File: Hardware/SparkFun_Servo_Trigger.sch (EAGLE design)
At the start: 30 parts, among them U1 ATTINY84, Y1 16MHZ

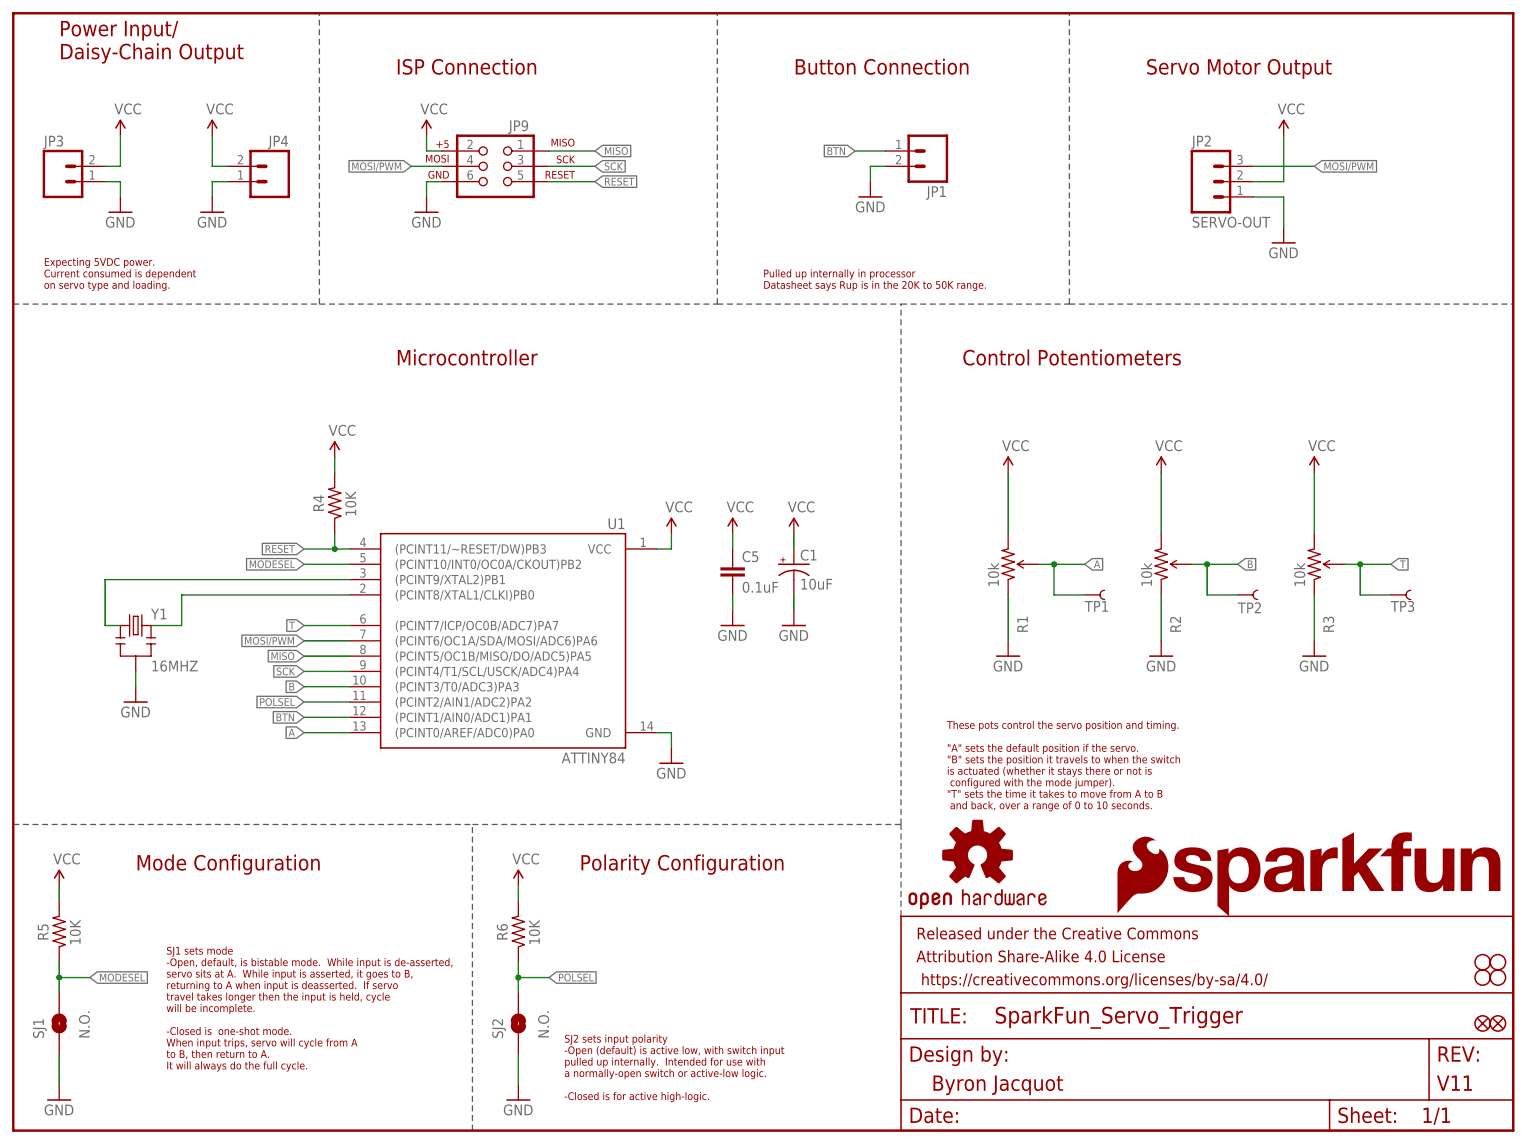
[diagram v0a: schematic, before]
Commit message: Updates from checklist.
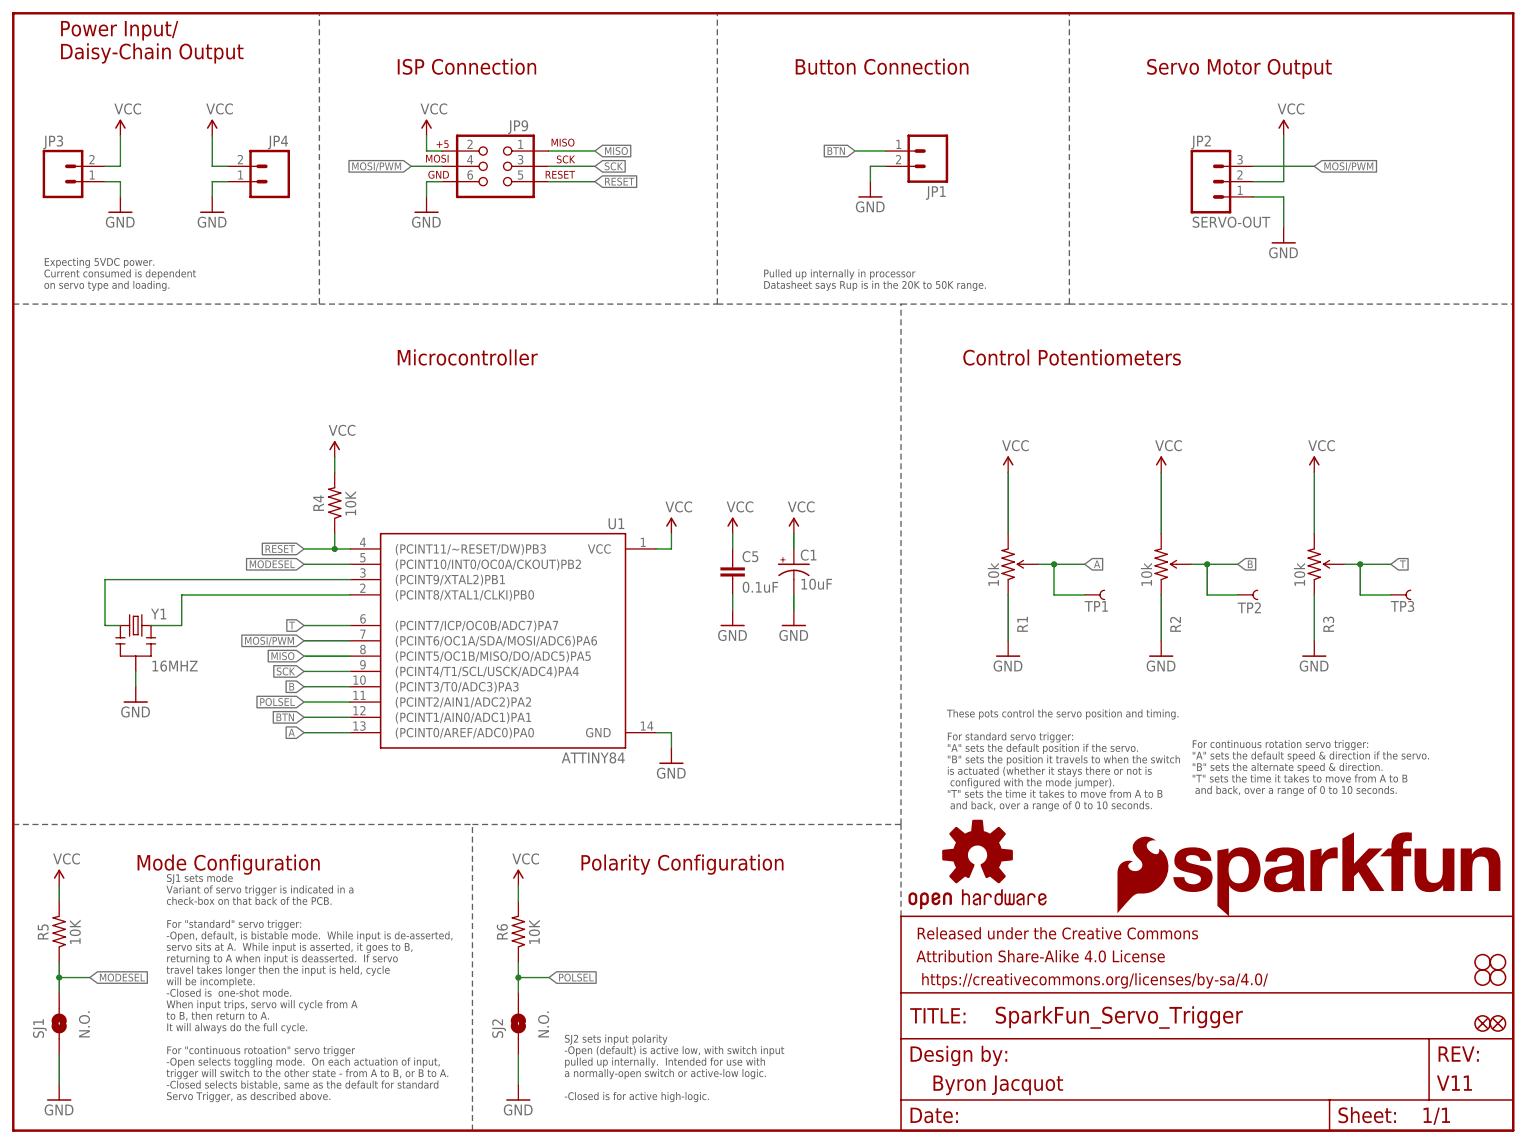
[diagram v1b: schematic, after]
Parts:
- FRAME1: value (none) -> frame
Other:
- note added: "For continuous rotation servo trigger: "A" sets the default speed & direction if the servo. "B" sets the alternate speed & direction. "T" sets the time it takes to move from A to B and back, over a range of 0 to 10 seconds."
- note added: "SJ1 sets mode Variant of servo trigger is indicated in a check-box on that back of the PCB. For "standard" servo trigger: -Open, default, is bistable mode. While input is de-asserted, servo sits at A. While input is asserted, it goes to B, returning to A when input is deasserted. If servo travel takes longer then the input is held, cycle will be incomplete. -Closed is one-shot mode. When input tr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"
- note added: "These pots control the servo position and timing. For standard servo trigger: "A" sets the default position if the servo. "B" sets the position it travels to when the switch is actuated (whether it stays there or not is configured with the mode jumper). "T" sets the time it takes to move from A to B and back, over a range of 0 to 10 seconds."
- note removed: "SJ1 sets mode -Open, default, is bistable mode. While input is de-asserted, servo sits at A. While input is asserted, it goes to B, returning to A when input is deasserted. If servo travel takes longer then the input is held, cycle will be incomplete. -Closed is one-shot mode. When input trips, servo will cycle from A to B, then return to A. It will always do the full cycle."
- note removed: "These pots control the servo position and timing. "A" sets the default position if the servo. "B" sets the position it travels to when the switch is actuated (whether it stays there or not is configured with the mode jumper). "T" sets the time it takes to move from A to B and back, over a range of 0 to 10 seconds."
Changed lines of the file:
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@@
 </classes>
 <parts>
-<part name="FRAME1" library="SparkFun-Aesthetics" deviceset="FRAME-LETTER" device="">
+<part name="FRAME1" library="SparkFun-Aesthetics" deviceset="FRAME-LETTER" device="" value="frame">
 <attribute name="DESIGNER" value="Byron Jacquot"/>
 <attribute name="VERSION" value="V11"/>
@@
 <text x="20.32" y="43.18" size="2.54" layer="94" font="vector">Mode Configuration</text>
 <text x="93.98" y="43.18" size="2.54" layer="94" font="vector">Polarity Configuration</text>
-<text x="25.4" y="10.16" size="1.27" layer="94">SJ1 sets mode
+<text x="25.4" y="5.08" size="1.27" layer="97">SJ1 sets mode
+Variant of servo trigger is indicated in a
+check-box on that back of the PCB.
+For "standard" servo trigger:
 -Open, default, is bistable mode.  While input is de-asserted,
 servo sits at A.  While input is asserted, it goes to B,
@@
 When input trips, servo will cycle from A
 to B, then return to A.
-It will always do the full cycle.</text>
-<text x="91.44" y="5.08" size="1.27" layer="94">SJ2 sets input polarity
+It will always do the full cycle.
+For "continuous rotoation" servo trigger
+-Open selects toggling mode.  On each actuation of input,
+trigger will switch to the other state - from A to B, or B to A.
+-Closed selects bistable, same as the default for standard
+Servo Trigger, as described above.</text>
+<text x="91.44" y="5.08" size="1.27" layer="97">SJ2 sets input polarity
 -Open (default) is active low, with switch input
 pulled up internally.  Intended for use with
 a normally-open switch or active-low logic.
 -Closed is for active high-logic.</text>
-<text x="124.46" y="139.7" size="1.27" layer="94">Pulled up internally in processor
+<text x="124.46" y="139.7" size="1.27" layer="97">Pulled up internally in processor
 Datasheet says Rup is in the 20K to 50K range.</text>
-<text x="5.08" y="139.7" size="1.27" layer="94">Expecting 5VDC power.
+<text x="5.08" y="139.7" size="1.27" layer="97">Expecting 5VDC power.
 Current consumed is dependent
 on servo type and loading.</text>
-<text x="154.94" y="53.34" size="1.27" layer="94">These pots control the servo position and timing.
+<text x="154.94" y="53.34" size="1.27" layer="97">These pots control the servo position and timing.
+For standard servo trigger:
 "A" sets the default position if the servo.
 "B" sets the position it travels to when the switch
@@
 "T" sets the time it takes to move from A to B
  and back, over a range of 0 to 10 seconds.</text>
+<text x="195.58" y="55.88" size="1.27" layer="97">For continuous rotation servo trigger:
+"A" sets the default speed &amp; direction if the servo.
+"B" sets the alternate speed &amp; direction.
+"T" sets the time it takes to move from A to B
+ and back, over a range of 0 to 10 seconds.</text>
